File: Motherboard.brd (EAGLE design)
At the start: 100 x 80 mm, 15 parts

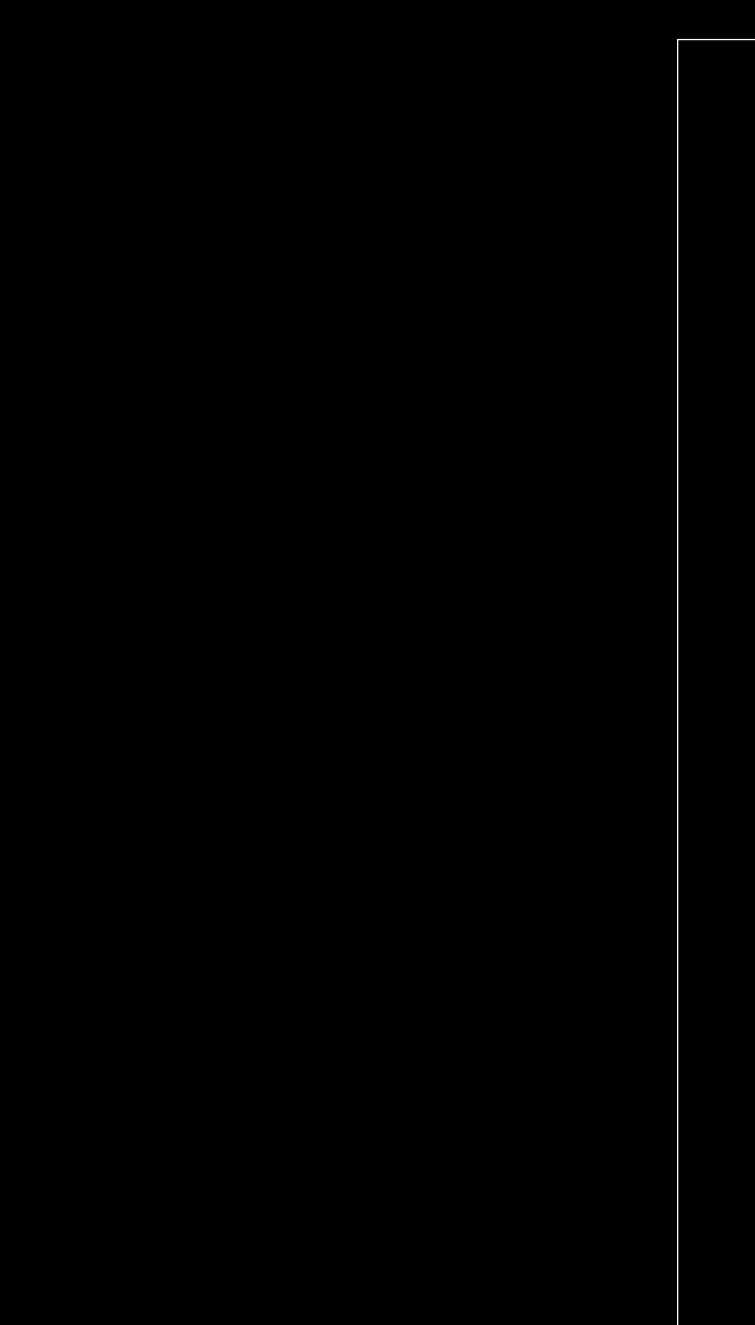
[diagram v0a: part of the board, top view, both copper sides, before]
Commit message: more circuit
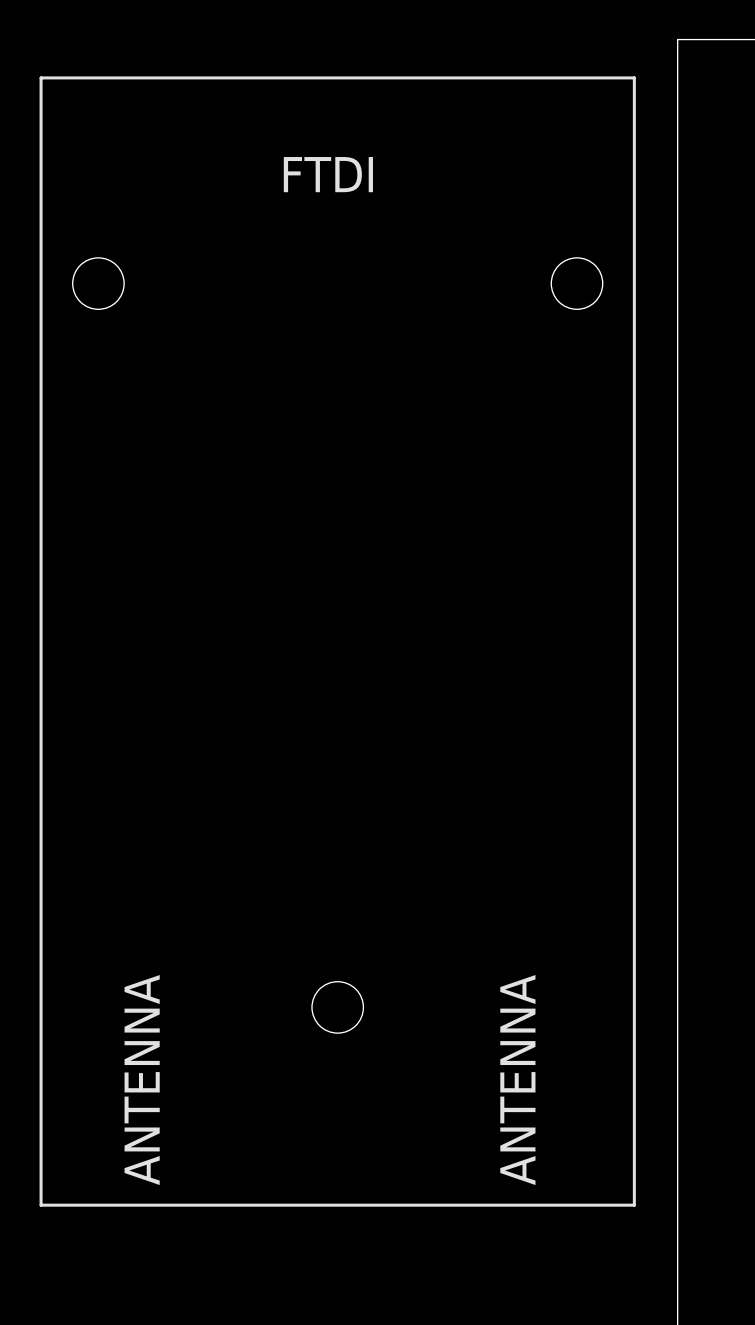
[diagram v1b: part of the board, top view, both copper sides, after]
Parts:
- added U$1: (no value), ArduinoNanoV30:RADIO
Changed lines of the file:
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@@
 <attribute name="SPICEPREFIX" value="R" x="91.44" y="5.08" size="1.778" layer="27" display="off"/>
 </element>
+<element name="U$1" library="ArduinoNanoV30" package="RADIO" value="" x="-17.78" y="49.53" rot="R90"/>
 </elements>
 <signals>
